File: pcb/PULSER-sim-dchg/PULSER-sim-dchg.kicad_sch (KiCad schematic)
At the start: 30 parts

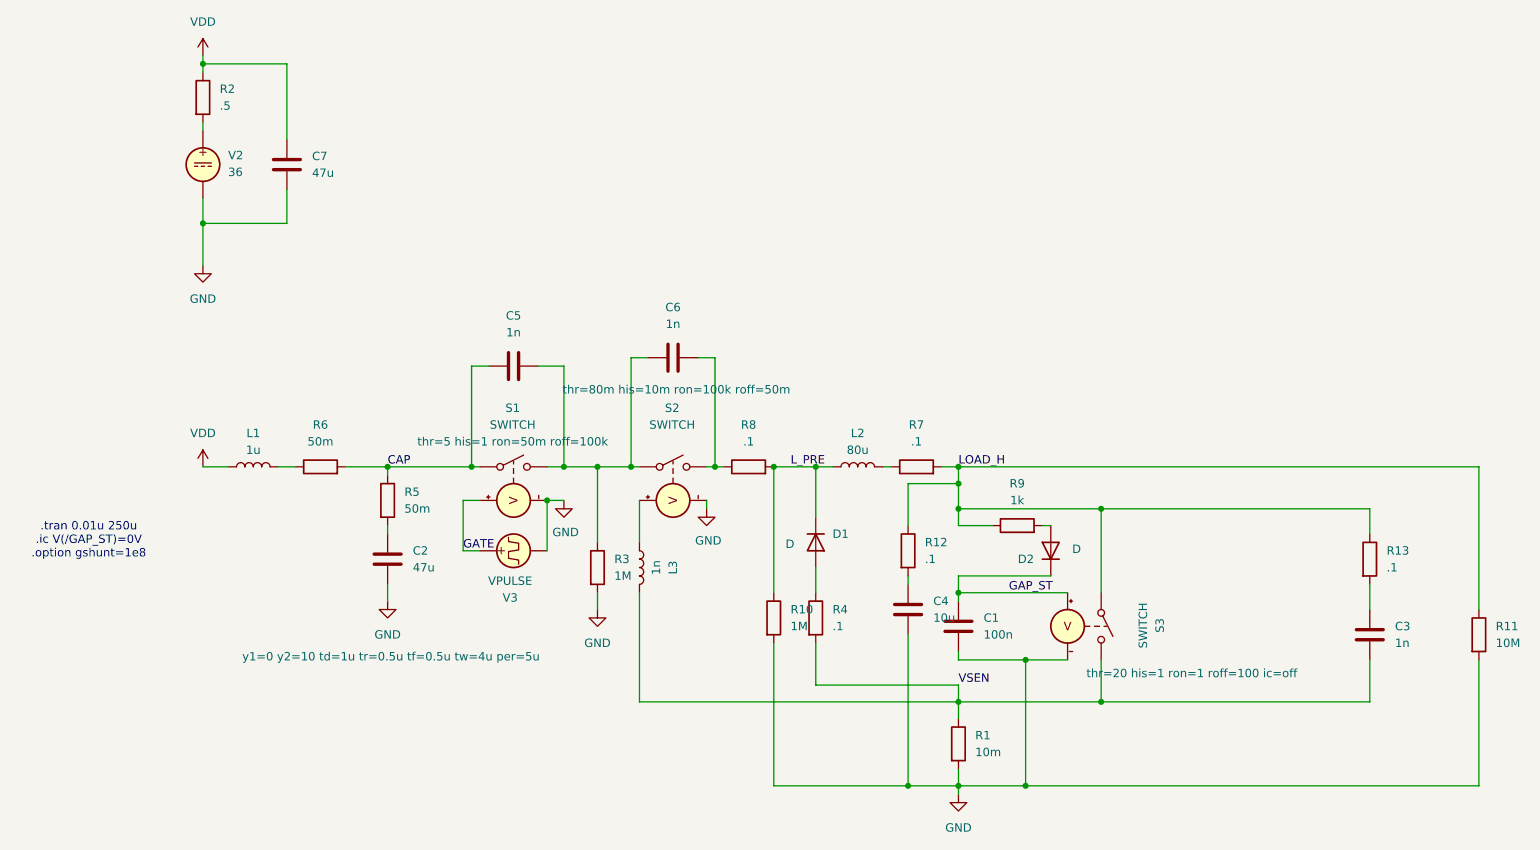
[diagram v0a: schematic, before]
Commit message: Upgrade KiCad & new discharge exps
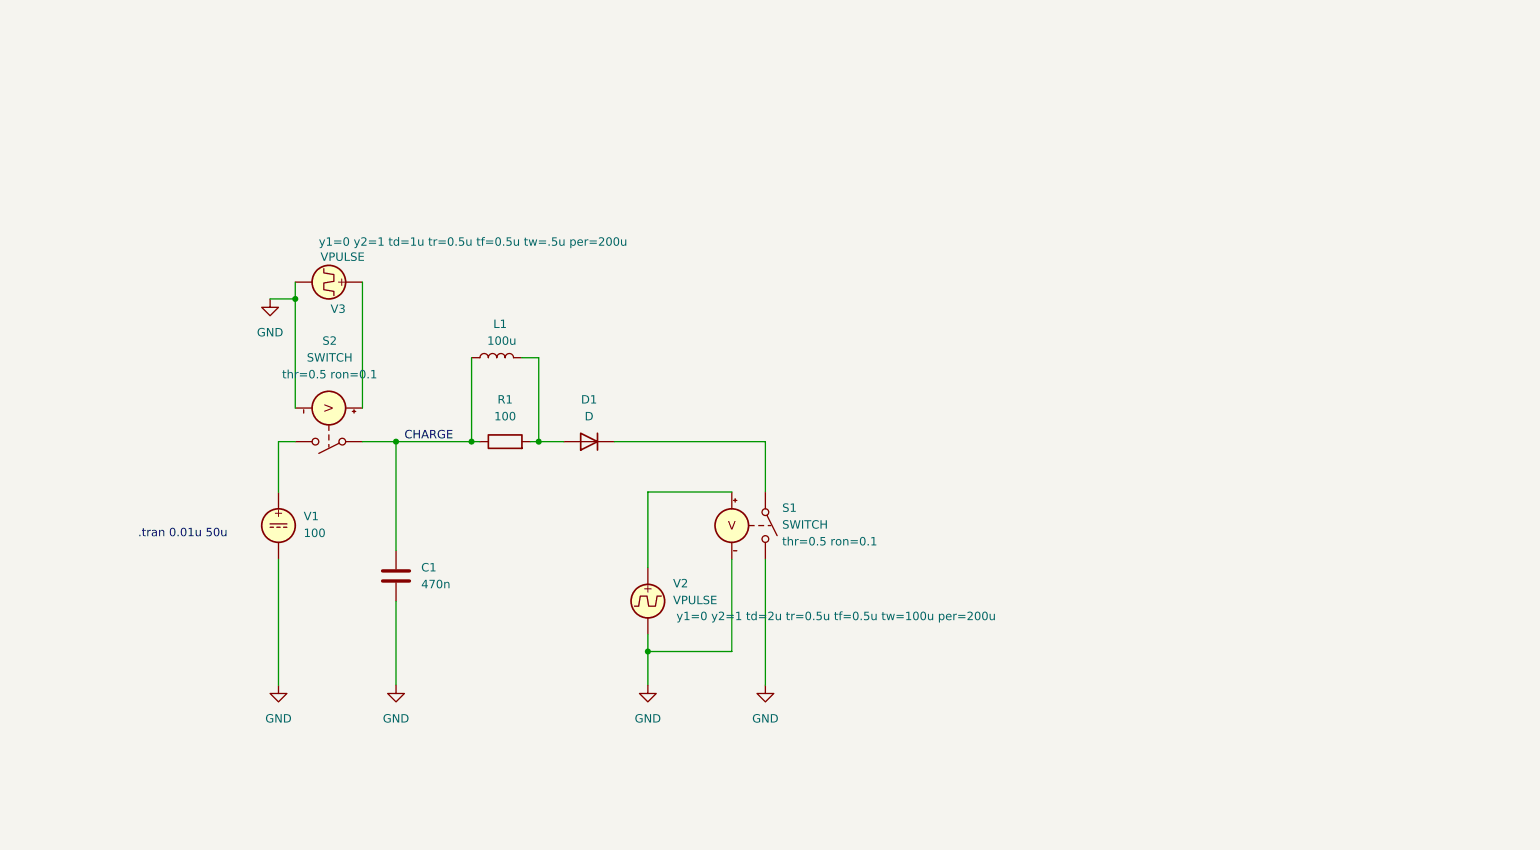
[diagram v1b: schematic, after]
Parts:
- removed C2, C7: 47u, symbol Device:C
- removed C3, C5, C6: 1n, symbol Device:C
- removed C4: 10u, symbol Device:C
- removed D2: D, symbol Device:D
- removed L2: 80u, symbol Device:L
- removed L3: 1n, symbol Device:L
- removed R10, R3: 1M, symbol Device:R
- removed R11: 10M, symbol Device:R
- removed R12, R13, R4, R7, R8: .1, symbol Device:R
- removed R2: .5, symbol Device:R
- removed R5, R6: 50m, symbol Device:R
- removed R9: 1k, symbol Device:R
- removed S3: SWITCH, symbol Simulation_SPICE:SWITCH
- removed V2: 36, symbol Simulation_SPICE:VDC
- added V1: 100, symbol Simulation_SPICE:VDC
- added V2: VPULSE, symbol Simulation_SPICE:VPULSE
- C1: value 100n -> 470n
- L1: value 1u -> 100u
- R1: value 10m -> 100
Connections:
- net GAP_ST is gone; now on net GND: C1.2
- net L_PRE is gone; now on an unnamed net: D1.1 (K)
- net VDD is gone; now on net CHARGE: L1.1
- net VSEN is gone; now on net CHARGE: R1.1
- net GND: now also S1.2 (N-), V1.2, V2.2; no longer C1.1, R1.2
- net CHARGE: now reaches S2.1 (N+)
- net CHARGE: now also C1.1; no longer S1.2 (N-)
- net at L1.2: now also D1.2 (A), R1.2
- net at S2.3 (C+): now also V3.1
- net at S2.2 (N-): now also V1.1
- net CAP: no longer names the net of S1.1 (N+)
- net GATE: no longer names the net of S1.3 (C+)
- net GATE: now also V2.1; no longer V3.1
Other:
- note added: ".tran 0.01u 50u"
- note removed: ".tran 0.01u 250u .ic V(/GAP_ST)=0V .option gshunt=1e8"
